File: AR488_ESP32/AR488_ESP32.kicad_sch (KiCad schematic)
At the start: 22 parts, among them J1 GPIB_24, J2 DC_7-12V, J3 SHIELD, Q1 AO3401A, Q2 AO3401A, Q3 MMBT5551L, U1 Heltec_WiFi_Kit_32_V2, U2 SN75160BDW, U3 SN75161BN, U4 MCP23017, U5 AMS1117-5.0

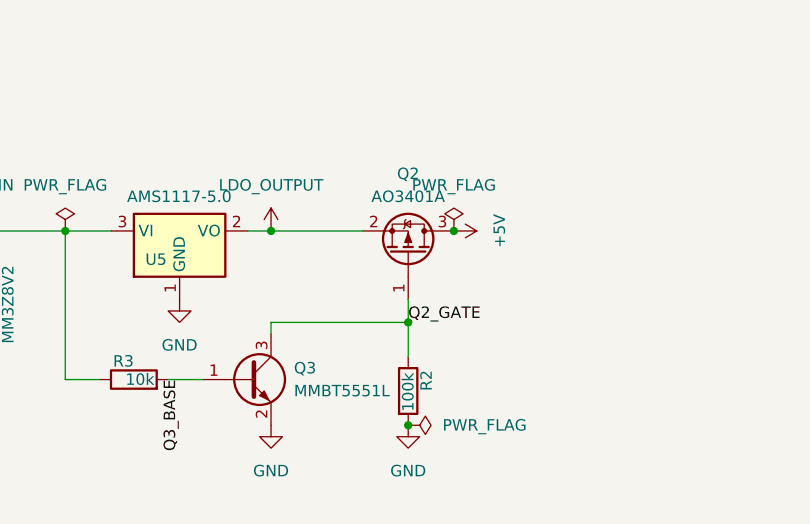
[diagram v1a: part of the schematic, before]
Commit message: feat: v1.1 — PCB and schematic updates, Elecrow manufacturing v1.1
Co-Authored-By: Claude Opus 4.6 <noreply@anthropic.com>
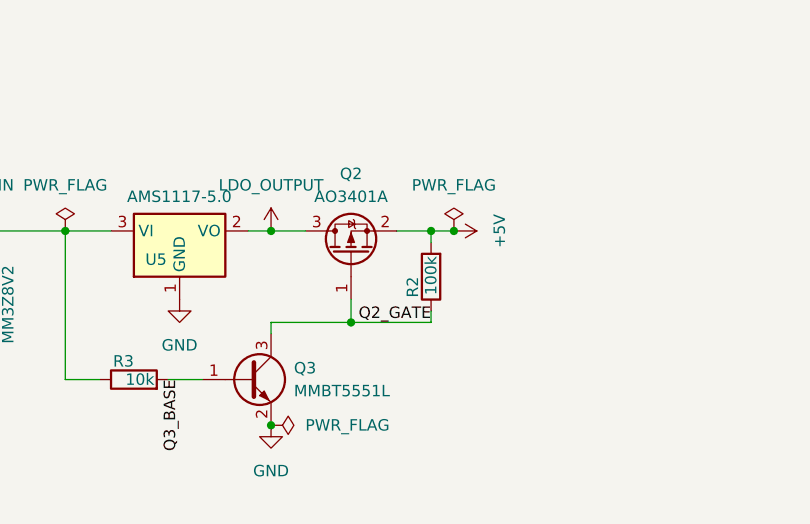
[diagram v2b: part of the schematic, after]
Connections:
- net +5V: now also Q2.2 (S), R2.2; no longer Q2.3 (D)
- net GND: no longer R2.2
- net LDO_OUTPUT: now also Q2.3 (D); no longer Q2.2 (S)
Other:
- moved on the sheet: Q2, R2
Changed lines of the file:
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@@
 		(title "AR488_ESP32")
 		(date "2026-04-11")
-		(rev "1.0")
+		(rev "1.1")
 		(comment 1 "AR-488 GPIB Interface for Tektronix TDS784A")
 		(comment 3 "Generated by circuit-synth and modified by author")
@@
 	)
 	(junction
-		(at 143.51 177.8)
-		(diameter 0)
-		(color 0 0 0 0)
-	)
-	(junction
 		(at 105.41 156.21)
 		(diameter 0)
@@
 	)
 	(junction
+		(at 128.27 177.8)
+		(diameter 0)
+		(color 0 0 0 0)
+	)
+	(junction
+		(at 146.05 156.21)
+		(diameter 0)
+		(color 0 0 0 0)
+	)
+	(junction
 		(at 128.27 156.21)
 		(diameter 0)
@@
 	)
 	(junction
-		(at 143.51 166.37)
+		(at 137.16 166.37)
 		(diameter 0)
 		(color 0 0 0 0)
@@
 	(wire
 		(pts
+			(xy 146.05 156.21) (xy 148.59 156.21)
+		)
+		(stroke
+			(width 0)
+			(type default)
+		)
+	)
+	(wire
+		(pts
+			(xy 146.05 156.21) (xy 146.05 157.48)
+		)
+		(stroke
+			(width 0)
+			(type default)
+		)
+	)
+	(wire
+		(pts
+			(xy 142.24 156.21) (xy 146.05 156.21)
+		)
+		(stroke
+			(width 0)
+			(type default)
+		)
+	)
+	(wire
+		(pts
 			(xy 55.88 156.21) (xy 67.31 156.21)
 		)
@@
 	(wire
 		(pts
-			(xy 128.27 156.21) (xy 138.43 156.21)
+			(xy 128.27 156.21) (xy 132.08 156.21)
 		)
 		(stroke
@@
 	(wire
 		(pts
-			(xy 143.51 166.37) (xy 128.27 166.37)
+			(xy 137.16 166.37) (xy 146.05 166.37)
 		)
 		(stroke
@@
 	(wire
 		(pts
-			(xy 143.51 163.83) (xy 143.51 166.37)
+			(xy 137.16 166.37) (xy 128.27 166.37)
 		)
 		(stroke
@@
 	(wire
 		(pts
-			(xy 143.51 166.37) (xy 143.51 170.18)
+			(xy 137.16 163.83) (xy 137.16 166.37)
+		)
+		(stroke
+			(width 0)
+			(type default)
+		)
+	)
+	(wire
+		(pts
+			(xy 146.05 166.37) (xy 146.05 165.1)
 		)
 		(stroke
@@
 	)
 	(label "Q2_GATE"
-		(at 143.51 166.37 0)
+		(at 146.05 166.37 180)
 		(effects
 			(font
 				(size 1.27 1.27)
 			)
-			(justify left bottom)
+			(justify right bottom)
 		)
 	)
@@
 	(symbol
 		(lib_id "power:PWR_FLAG")
-		(at 143.51 177.8 270)
+		(at 128.27 177.8 270)
 		(unit 1)
 		(exclude_from_sim no)
@@
 		(fields_autoplaced yes)
 		(property "Reference" "#FLG03"
-			(at 145.415 177.8 0)
+			(at 130.175 177.8 0)
 			(effects
 				(font
@@
 		)
 		(property "Value" "PWR_FLAG"
-			(at 147.32 177.7999 90)
+			(at 132.08 177.7999 90)
 			(effects
 				(font
@@
 		)
 		(property "Footprint" ""
-			(at 143.51 177.8 0)
+			(at 128.27 177.8 0)
 			(effects
 				(font
@@
 		)
 		(property "Datasheet" "~"
-			(at 143.51 177.8 0)
+			(at 128.27 177.8 0)
 			(effects
 				(font
@@
 		)
 		(property "Description" "Special symbol for telling ERC where power comes from"
-			(at 143.51 177.8 0)
+			(at 128.27 177.8 0)
 			(effects
 				(font
@@
 	(symbol
 		(lib_id "Transistor_FET:AO3401A")
-		(at 143.51 158.75 270)
-		(mirror x)
+		(at 137.16 158.75 90)
 		(unit 1)
 		(exclude_from_sim no)
@@
 		(dnp no)
 		(property "Reference" "Q2"
-			(at 143.51 149.86 90)
+			(at 137.16 149.86 90)
 			(effects
 				(font
@@
 		)
 		(property "Value" "AO3401A"
-			(at 143.51 152.4 90)
+			(at 137.16 152.4 90)
 			(effects
 				(font
@@
 		)
 		(property "Footprint" "Package_TO_SOT_SMD:SOT-23"
-			(at 141.605 153.67 0)
+			(at 139.065 153.67 0)
 			(effects
 				(font
@@
 		)
 		(property "Datasheet" "http://www.aosmd.com/pdfs/datasheet/AO3401A.pdf"
-			(at 139.7 153.67 0)
+			(at 140.97 153.67 0)
 			(effects
 				(font
@@
 		)
 		(property "Description" "-4.0A Id, -30V Vds, P-Channel MOSFET, SOT-23"
-			(at 143.51 158.75 0)
+			(at 137.16 158.75 0)
 			(effects
 				(font
@@
 	(symbol
 		(lib_id "Device:R")
-		(at 143.51 173.99 0)
+		(at 146.05 161.29 180)
 		(unit 1)
 		(exclude_from_sim no)
@@
 		(dnp no)
 		(property "Reference" "R2"
-			(at 145.542 173.99 90)
+			(at 144.018 161.29 90)
 			(effects
 				(font
@@
 		)
 		(property "Value" "100k"
-			(at 143.51 176.276 90)
+			(at 146.05 159.004 90)
 			(effects
 				(font
@@
 		)
 		(property "Footprint" "Resistor_SMD:R_0603_1608Metric"
-			(at 141.732 173.99 90)
+			(at 147.828 161.29 90)
 			(effects
 				(font
@@
 		)
 		(property "Datasheet" ""
-			(at 143.51 173.99 0)
+			(at 146.05 161.29 0)
 			(effects
 				(font
@@
 		)
 		(property "Description" ""
-			(at 143.51 173.99 0)
+			(at 146.05 161.29 0)
 			(effects
 				(font
@@
 		)
 		(property "hierarchy_path" "/9abb8f01-95c2-4415-84b9-c2d85c9cb37e"
-			(at 146.05 179.0699 0)
+			(at 143.51 156.2101 0)
 			(effects
 				(font
@@
 		)
 		(property "project_name" "AR488_ESP32"
-			(at 146.05 179.0699 0)
+			(at 143.51 156.2101 0)
 			(effects
 				(font
@@
 		)
 		(property "root_uuid" "9abb8f01-95c2-4415-84b9-c2d85c9cb37e"
-			(at 146.05 179.0699 0)
+			(at 143.51 156.2101 0)
 			(effects
 				(font
@@
 					(unit 1)
 				)
-			)
-		)
-	)
-	(symbol
-		(lib_id "power:GND")
-		(at 143.51 177.8 0)
-		(unit 1)
-		(exclude_from_sim no)
-		(in_bom yes)
-		(on_board yes)
-		(dnp no)
-		(property "Reference" "#PWR01"
-			(at 143.51 171.45 0)
-			(effects
-				(font
-					(size 1.27 1.27)
-				)
-				(justify left)
-				(hide yes)
-			)
-		)
-		(property "Value" "GND"
-			(at 143.51 182.88 0)
-			(effects
-				(font
-					(size 1.27 1.27)
-				)
-			)
-		)
-		(property "Footprint" ""
-			(at 143.51 177.8 0)
-			(effects
-				(font
-					(size 1.27 1.27)
-				)
-				(hide yes)
-			)
-		)
-		(property "Datasheet" ""
-			(at 143.51 177.8 0)
-			(effects
-				(font
-					(size 1.27 1.27)
-				)
-			)
-		)
-		(property "Description" ""
-			(at 143.51 177.8 0)
-			(effects
-				(font
-					(size 1.27 1.27)
-				)
-			)
-		)
-		(pin "1"
-		)
-		(instances
-			(project "AR488_ESP32"
-				(path "/9abb8f01-95c2-4415-84b9-c2d85c9cb37e"
-					(reference "#PWR01")
-					(unit 1)
-				)
